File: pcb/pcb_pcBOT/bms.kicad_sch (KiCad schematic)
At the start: 23 parts, among them J201 Lipo, U201 BQ25896RTW

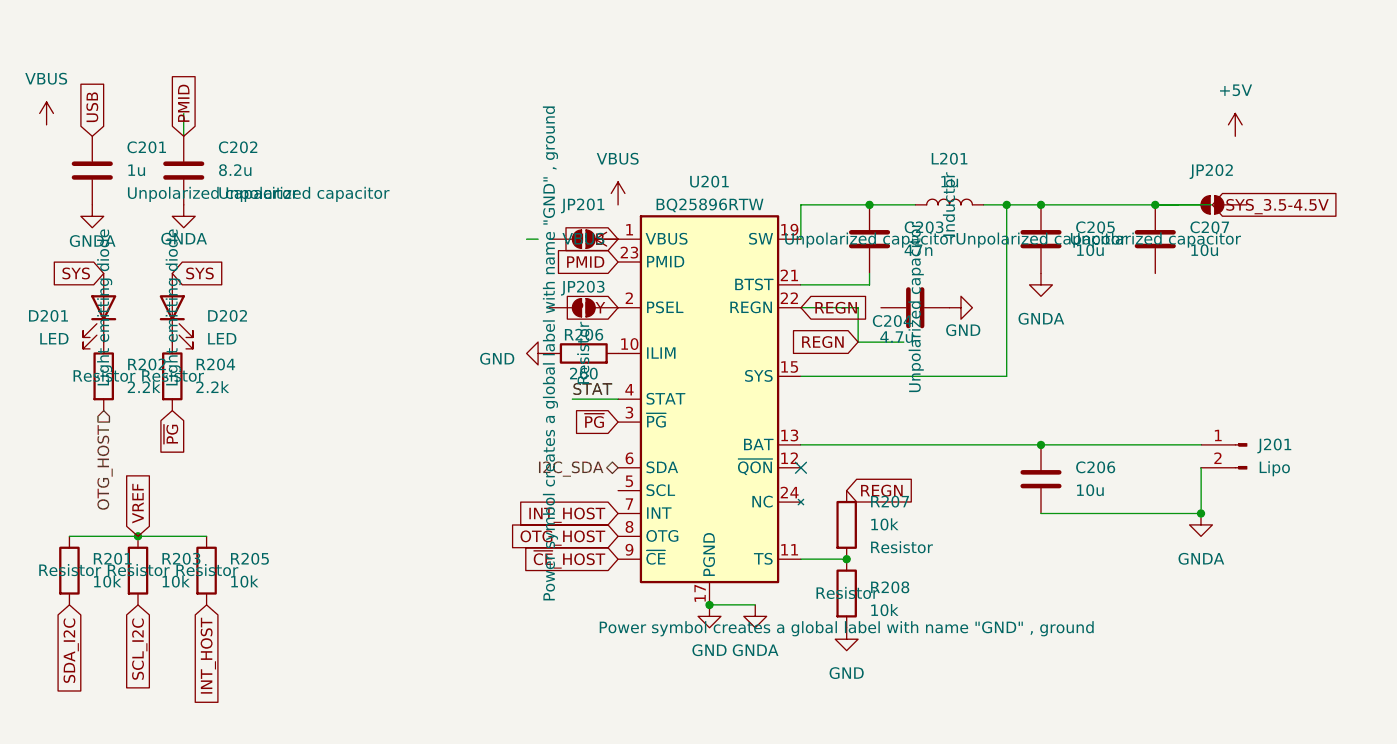
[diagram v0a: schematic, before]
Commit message: manual merge
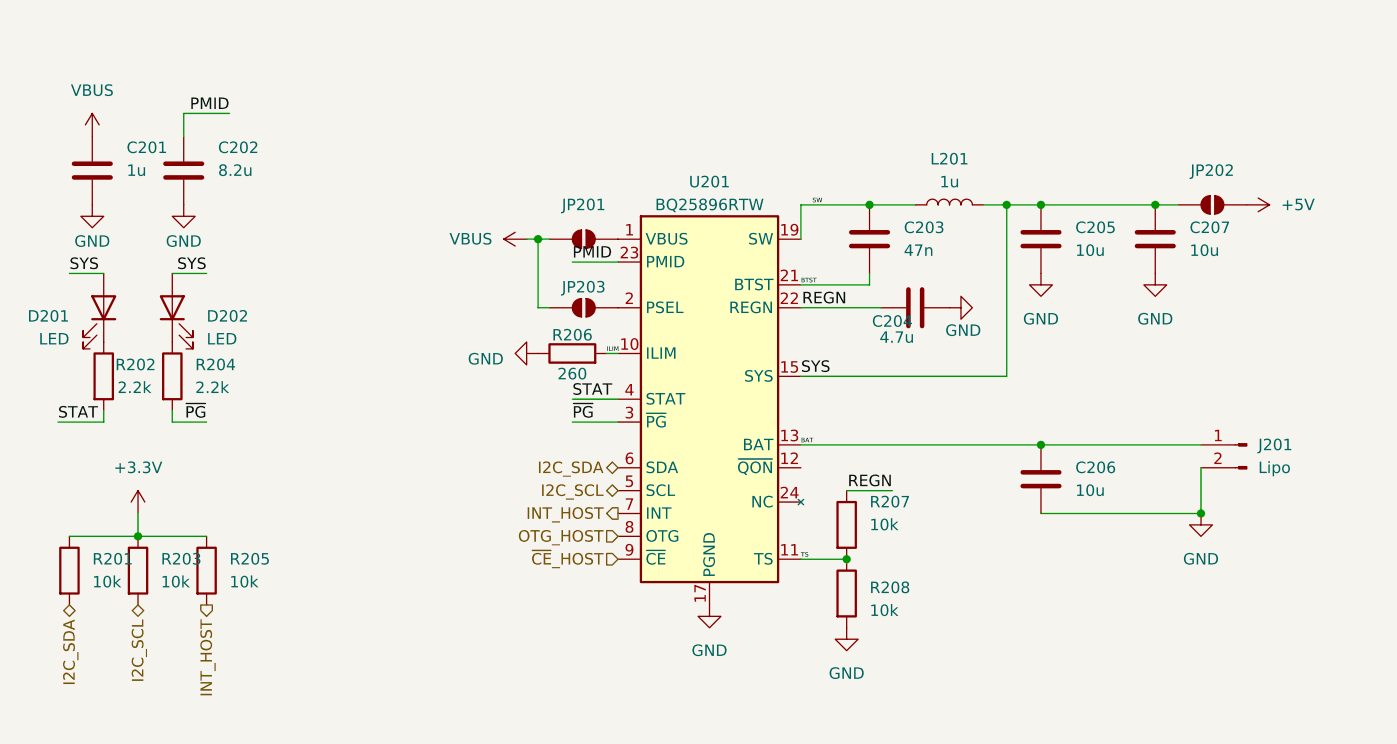
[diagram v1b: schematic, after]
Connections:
- net SCL_I2C is gone; now on net I2C_SCL: R203.2
- net SDA_I2C is gone; now on net I2C_SDA: R201.2
- net SYS_3.5-4.5V is gone; now on net SYS: C205.1, C207.1, JP202.1 (A), L201.2, U201.15 (SYS), U201.16 (SYS)
- net +5V: now also JP202.2 (B)
- net GND: now also C207.2
- net OTG_HOST: no longer R202.2
- net REGN: now also C204.2
- net STAT: now also R202.2
- net VBUS: now also JP201.1 (A), JP203.1 (A); no longer JP201.2 (B), U201.1 (VBUS)
- net SW: now reaches C203.1, L201.1, U201.19 (SW), U201.20 (SW)
- net BTST: now reaches C203.2, U201.21 (BTST)
- net BAT: now reaches C206.1, J201.1 (Pin_1), U201.13 (BAT), U201.14 (BAT)
- net TS: now reaches R207.2, R208.1, U201.11 (TS)
- net ILIM: now reaches R206.2, U201.10 (ILIM)
- net I2C_SCL: now reaches U201.5 (SCL)
- net PHY: no longer names the net of JP203.2 (B), U201.2 (PSEL)
- net VREF renamed +3.3V
- new net: JP201.2 (B), U201.1 (VBUS)
- no-connect marks 1 -> 0
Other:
- moved on the sheet: R206
